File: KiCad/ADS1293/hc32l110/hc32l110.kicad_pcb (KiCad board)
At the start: 4 copper layers, 22 x 18.5 mm, 34 parts, among them J1 COM_IN, J2 COM_OUT, U1 ADS1293CISQE-NOPB, U2 HC32L110C6UA

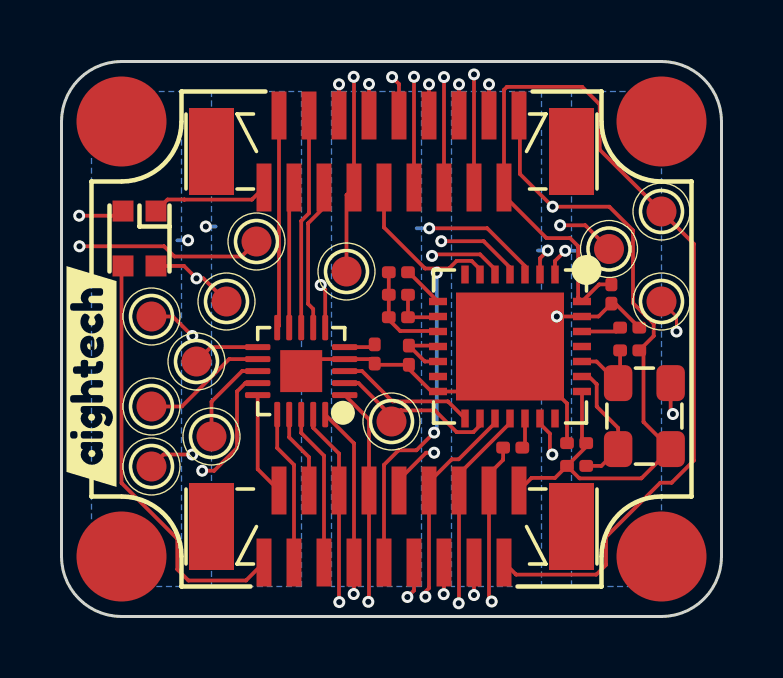
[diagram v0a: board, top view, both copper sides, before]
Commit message: updated
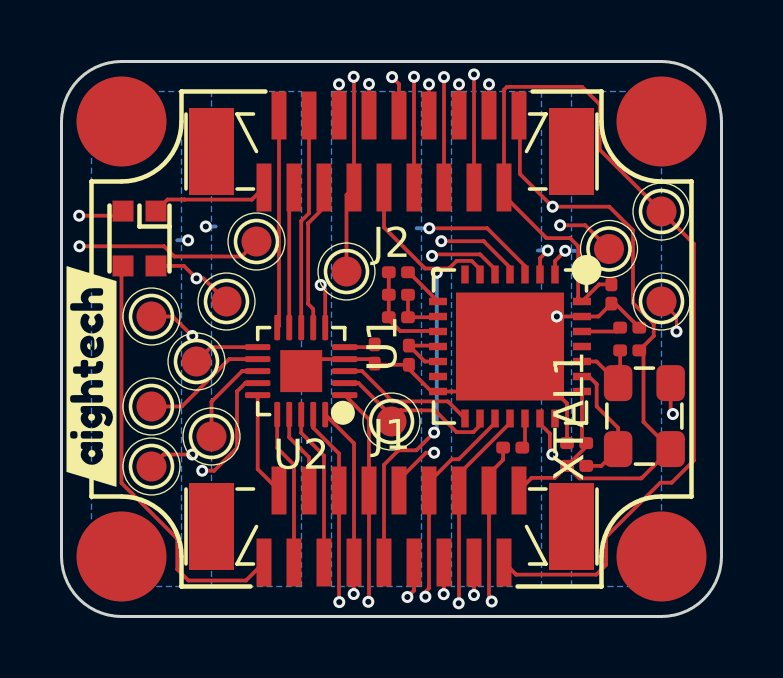
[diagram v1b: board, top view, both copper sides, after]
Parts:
- J1, J2: footprint 00_Custom:XF2J-1824-12A -> 00_custom-footprints:XF2J-1824-12A
- LED1: footprint 00_Custom:WS2812-2020 -> 00_custom-footprints:WS2812-2020
- U1: footprint 00_Custom:ADS1293CISQE -> 00_custom-footprints:ADS1293CISQE
- U2: footprint 00_Custom:QFN-20-1EP_3x3mm_P0.4mm_EP1.4x1.4mm -> 00_custom-footprints:QFN-20-1EP_3x3mm_P0.4mm_EP1.4x1.4mm
- XTAL1: footprint 00_Custom:SMD3225-4P -> 00_custom-footprints:SMD3225-4P

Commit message: lot of modification, preparing a refactor + some rendering
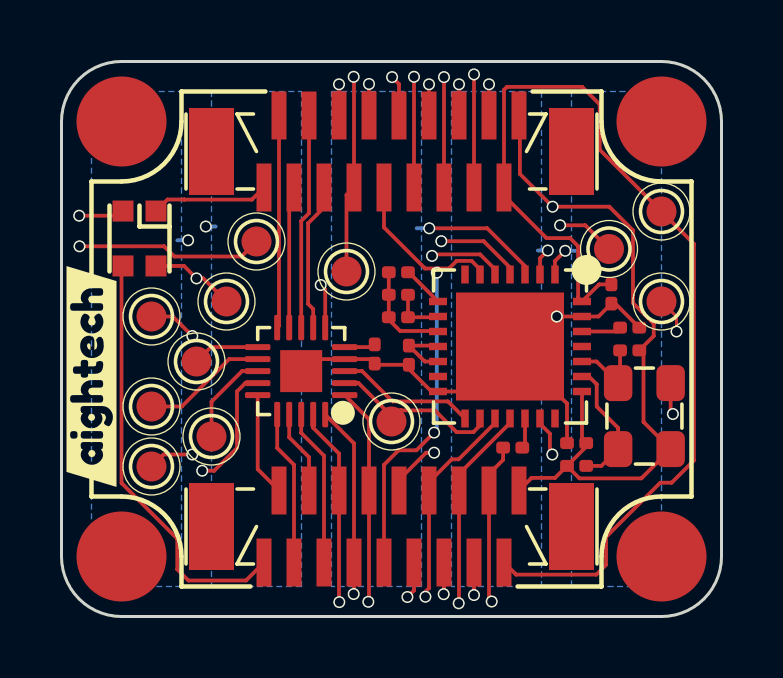
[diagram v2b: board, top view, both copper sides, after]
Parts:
- J1: value COM_IN -> XF2J-1824-12A
- J2: value COM_OUT -> XF2J-1824-12A
